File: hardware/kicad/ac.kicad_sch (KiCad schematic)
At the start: 25 parts, among them J1 AC_Input, J2 Hirose RPC1-12RB-6P(71), Q1 KIA50N06BD, Q2 KIA50N06BD, U1 VOS628A, U2 L78L24_SOT89, U3 Si8751, U4 AP2111H-3.3

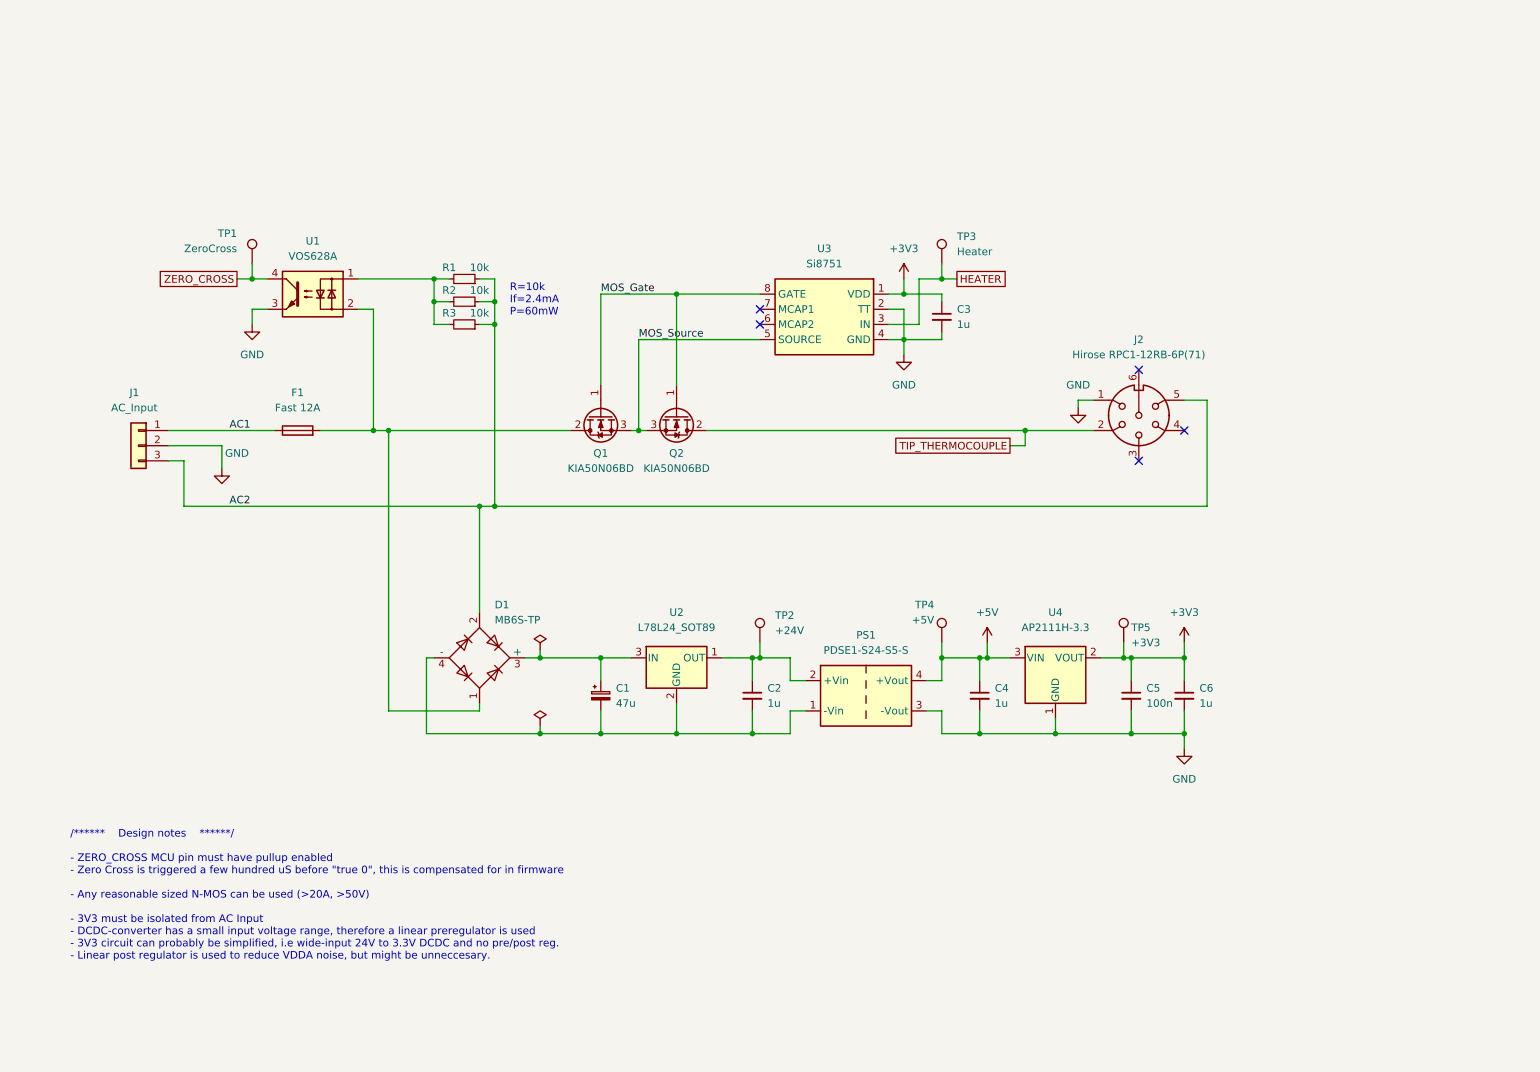
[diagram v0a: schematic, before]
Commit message: Schematic update.
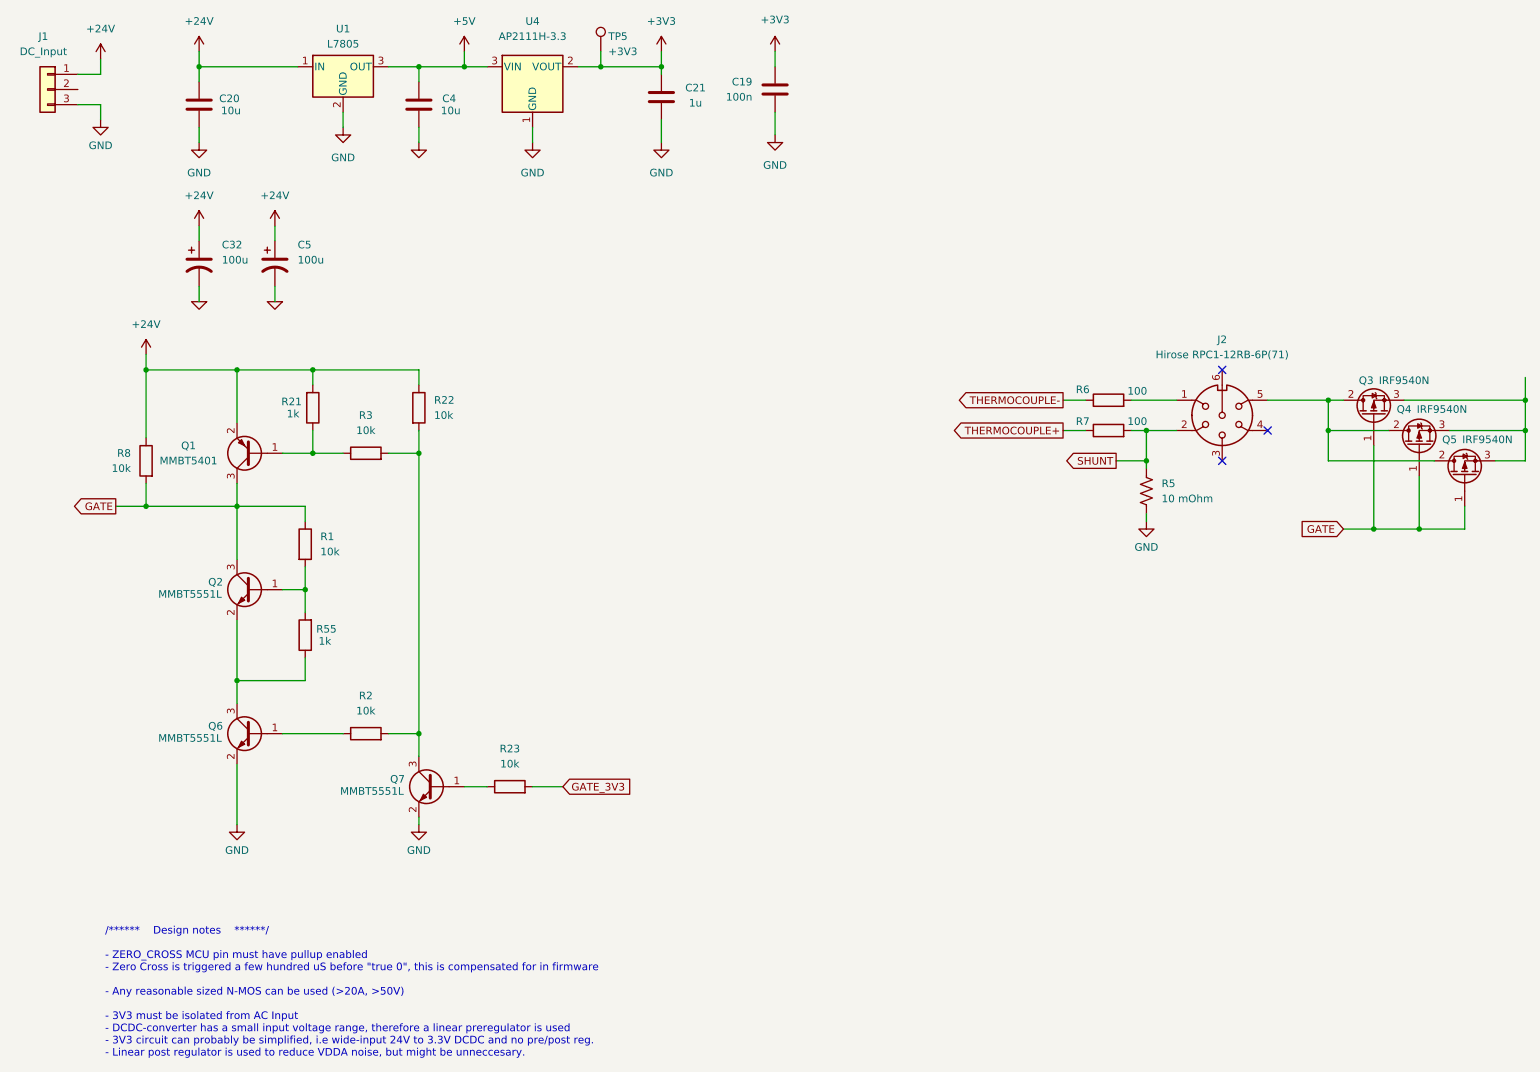
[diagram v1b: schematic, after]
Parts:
- removed C1: 47u, Capacitor_THT:CP_Radial_D8.0mm_P3.50mm, symbol Device:C_Polarized_Small
- removed C2, C3, C4, C6: 1u, Capacitor_SMD:C_1210_3225Metric, symbol Device:C_Small
- removed C5: 100n, Capacitor_SMD:C_0805_2012Metric, symbol Device:C_Small
- removed D1: MB6S-TP, Package_TO_SOT_SMD:TO-269AA, symbol 0_Howie:MB6S-TP
- removed F1: Fast 12A, Fuse:Fuseholder_Cylinder-5x20mm_Schurter_0031_8201_Horizontal_Open, symbol Device:Fuse
- removed PS1: PDSE1-S24-S5-S, 0_Howie:PDSE1_DCDC, symbol 0_Howie:PDSE1-S24-S5-S
- removed Q1, Q2: KIA50N06BD, Package_TO_SOT_SMD:TO-252-2, symbol 0_Howie:KIA50N06BD
- removed R1, R2, R3: 10k, Resistor_SMD:R_0805_2012Metric, symbol Device:R_Small
- removed TP1: ZeroCross, TestPoint:TestPoint_Pad_D1.0mm, symbol 0_Howie:TestPoint_D1_Pad
- removed TP2: +24V, TestPoint:TestPoint_Pad_D1.0mm, symbol 0_Howie:TestPoint_D1_Pad
- removed TP3: Heater, TestPoint:TestPoint_Pad_D1.0mm, symbol 0_Howie:TestPoint_D1_Pad
- removed TP4: +5V, TestPoint:TestPoint_Pad_D1.0mm, symbol 0_Howie:TestPoint_D1_Pad
- removed U1: VOS628A, Package_SO:SOP-4_4.4x2.6mm_P1.27mm, symbol 0_Howie:VOS628A
- removed U2: L78L24_SOT89, Package_TO_SOT_SMD:SOT-89-3, symbol Regulator_Linear:L78L24_SOT89
- removed U3: Si8751, Package_SO:SOIC-8_3.9x4.9mm_P1.27mm, symbol 0_Howie:Si8751
- added C19: 100n, Capacitor_SMD:C_0603_1608Metric_Pad1.08x0.95mm_HandSolder, symbol Device:C
- added C20, C4: 10u, Capacitor_SMD:C_0603_1608Metric_Pad1.08x0.95mm_HandSolder, symbol Device:C
- added C21: 1u, Capacitor_SMD:C_0603_1608Metric_Pad1.08x0.95mm_HandSolder, symbol Device:C
- added C32, C5: 100u, Capacitor_THT:CP_Radial_D8.0mm_P3.50mm, symbol solar_push_pull_sym_lib:UCY2V220MPD9TD
- added Q1: MMBT5401, Package_TO_SOT_SMD:SOT-23, symbol Transistor_BJT:MMBT3906
- added Q2, Q6, Q7: MMBT5551L, Package_TO_SOT_SMD:SOT-23, symbol Transistor_BJT:MMBT5551L
- added Q3, Q4, Q5: IRF9540N, Package_TO_SOT_THT:TO-220-3_Vertical, symbol Transistor_FET:IRF9540N
- added R1, R2, R22, R23, R3, R8: 10k, Resistor_SMD:R_0603_1608Metric_Pad0.98x0.95mm_HandSolder, symbol Device:R
- added R21, R55: 1k, Resistor_SMD:R_0603_1608Metric_Pad0.98x0.95mm_HandSolder, symbol Device:R
- added R5: 10 mOhm, Resistor_SMD:R_2512_6332Metric_Pad1.40x3.35mm_HandSolder, symbol Device:R_US
- added R6, R7: 100, Resistor_SMD:R_0603_1608Metric_Pad0.98x0.95mm_HandSolder, symbol Device:R
- added U1: L7805, Package_TO_SOT_THT:TO-220-3_Vertical, symbol Regulator_Linear:L7805
- J1: value AC_Input -> DC_Input
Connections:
- net +3V3: now also C19.2, C21.1
- net +5V: now also C4.1, U1.3 (OUT)
- net GND: now also J1.3 (Pin_3), C19.1, C20.2, C21.2, C4.2, Q6.2 (E), Q7.2 (E), R5.2, U1.2 (GND); no longer J1.2 (Pin_2), J2.1
- net AC1 renamed +24V
- net +24V: now also C20.1, C32.1, C5.1, Q1.2 (E), R21.2, R22.1, R8.1, U1.1 (IN)
- net AC2: no longer names the net of J2.5
- net AC2: now also Q3.2 (D), Q4.2 (D), Q5.2 (D); no longer J1.3 (Pin_3)
- net TIP_THERMOCOUPLE renamed SHUNT
- net SHUNT: now also R5.1, R7.2
- new net: Q3.3 (S), Q4.3 (S), Q5.3 (S)
- new net: Q2.1 (B), R1.2, R55.2
- new net: Q2.2 (E), Q6.3 (C), R55.1
- new net: J2.1, R6.2
- new net: Q1.1 (B), R21.1, R3.1
- new net: Q7.1 (B), R23.1
- new net: Q7.3 (C), R2.2, R22.2, R3.2
- new net: Q6.1 (B), R2.1
- new net 0: C32.2, C5.2
- new net GATE: Q1.3 (C), Q2.3 (C), Q3.1 (G), Q4.1 (G), Q5.1 (G), R1.1, R8.2
- new net GATE_3V3: R23.2
- new net THERMOCOUPLE+: R7.1
- new net THERMOCOUPLE-: R6.1
- no-connect marks 5 -> 3
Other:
- note removed: "R=10k If=2.4mA P=60mW"
- moved on the sheet: J1, J2, TP5, U4
